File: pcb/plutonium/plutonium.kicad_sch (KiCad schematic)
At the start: 43 parts, among them J1 Conn_01x04, J2 Conn_01x04, K1 diode-choc, K10 diode-choc, K11 diode-choc, K12 diode-choc, K13 diode-choc, K14 diode-choc, K15 diode-choc, K16 diode-choc, K17 diode-choc, K18 diode-choc, K19 diode-choc, K2 diode-choc, K20 diode-choc, K21 diode-choc, K22 diode-choc, K23 diode-choc, K24 diode-choc, K25 diode-choc, K26 diode-choc, K27 diode-choc, K28 diode-choc, K29 diode-choc, K3 diode-choc, K30 diode-choc, K4 diode-choc, K5 diode-choc, K6 diode-choc, K7 diode-choc, K8 diode-choc, K9 diode-choc, U1 xiao-ble, U2 xiao-ble, U3 MT25QL128ABA1ESE

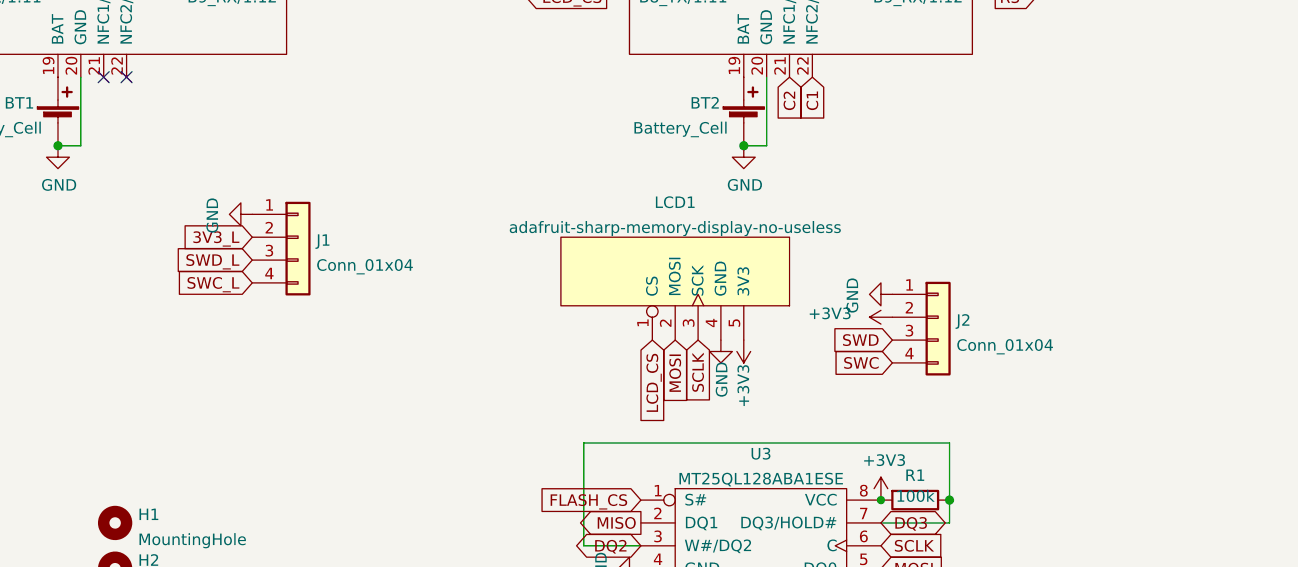
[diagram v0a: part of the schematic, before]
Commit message: [pcb] Plutonium: first revision
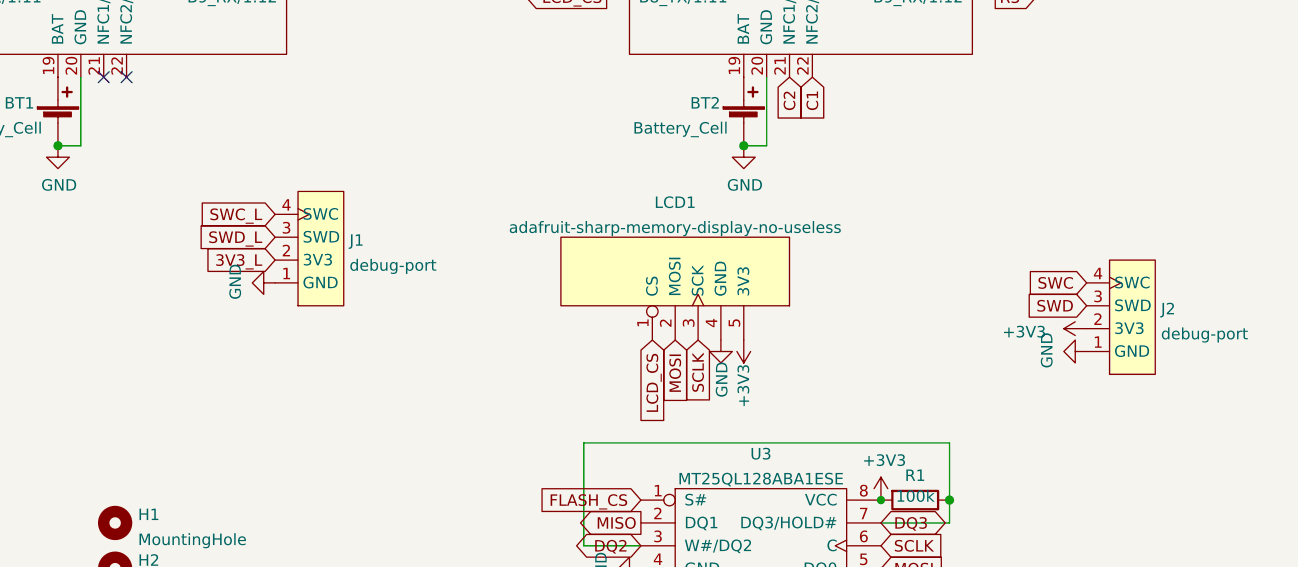
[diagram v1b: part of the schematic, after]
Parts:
- removed J1, J2: Conn_01x04, keeb-libs:debug-port-single-side, symbol Connector_Generic:Conn_01x04
- added J1, J2: debug-port, misc:debug-port-single-side, symbol misc:debug-port
- U1: footprint xiao:xiao-ble-smd -> xiao:xiao-ble-smd-cutout
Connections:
- net +3V3: now also J2.2 (3V3)
- net 3V3_L: now also J1.2 (3V3)
- net GND: now also J1.1 (GND), J2.1 (GND)
- net SWC: now also J2.4 (SWC)
- net SWC_L: now also J1.4 (SWC)
- net SWD: now also J2.3 (SWD)
- net SWD_L: now also J1.3 (SWD)
